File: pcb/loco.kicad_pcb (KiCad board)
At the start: 4 copper layers, 69.5 x 29.3 mm, 87 parts, among them J1 POWER, J2 INPUT, J3 I2C, J4 UART, J5 TagConnect, J6 GPIO_A, J7 GPIO_B, J8 Motor1, J9 Motor2, U1 NCV8718, U2 STM32G041K8U, U3 M95512-DRMF3TGK, U4 STSPIN220, U5 STSPIN220

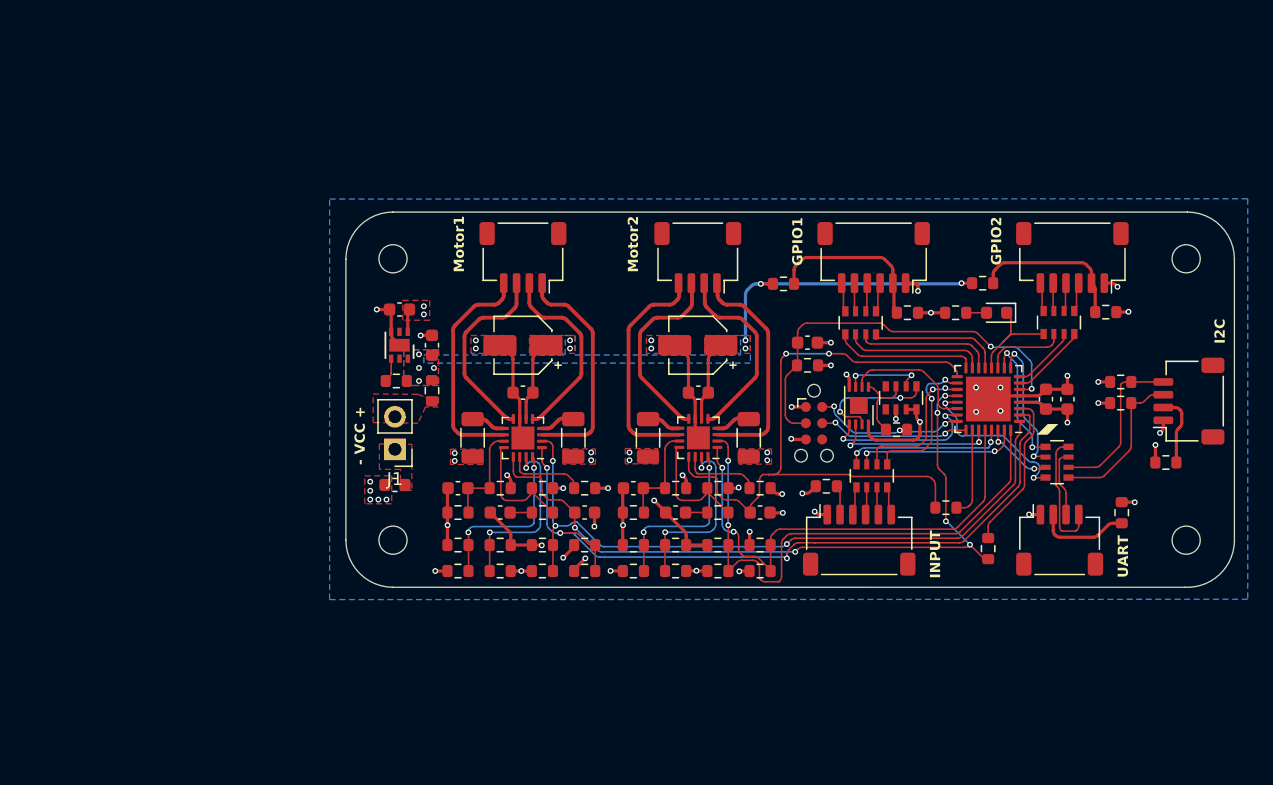
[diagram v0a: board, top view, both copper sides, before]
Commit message: pcb rev.0x03
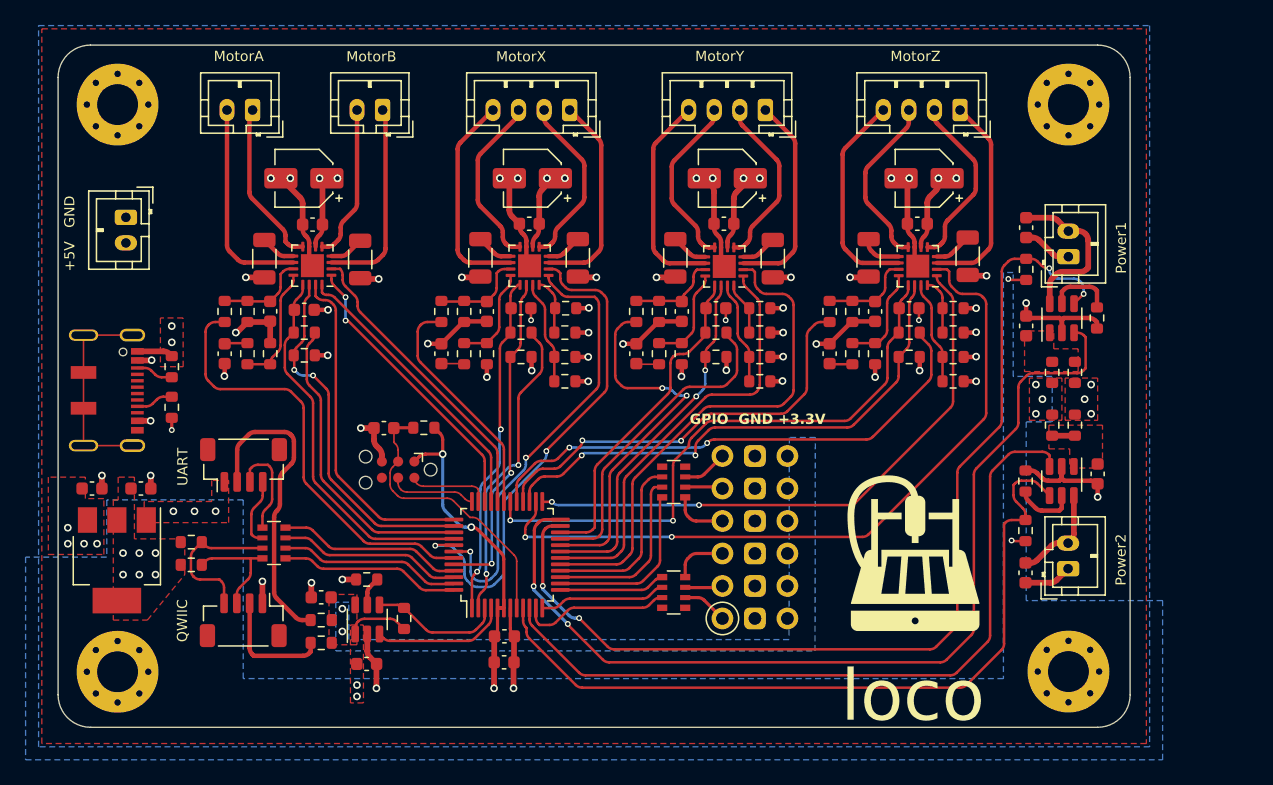
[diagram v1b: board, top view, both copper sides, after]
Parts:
- removed D1: LED, LED_SMD:LED_0603_1608Metric
- removed F1: Polyfuse, Fuse:Fuse_0603_1608Metric
- removed FB1, FB2, FB3, FB4, FB5, FB6: FerriteBead, Resistor_SMD:R_0603_1608Metric
- removed FB7, FB8: DNP, Resistor_SMD:R_0603_1608Metric
- removed J4: UART, Connector_JST:JST_SH_SM04B-SRSS-TB_1x04-1MP_P1.00mm_Horizontal
- removed J5: TagConnect, loco:Tag-Connect_TC2030-IDC-NL_2x03_P1.27mm_Vertical
- removed the REF** at (99.8, 56.3)
- removed RN4, RN5: 180Ω, Resistor_SMD:R_Array_Convex_4x0603
- added C16: 10uF, Capacitor_SMD:C_0603_1608Metric, F.Cu at (120.5, 59.1)
- added C17: 10uF, Capacitor_SMD:C_0603_1608Metric, F.Cu at (126.1, 70.7)
- added C18: 10uF, Capacitor_SMD:C_0603_1608Metric, F.Cu at (120.5, 51.4)
- added C19: 10uF, Capacitor_SMD:C_0603_1608Metric, F.Cu at (120.5, 78.4)
- added C20: 10uF, Capacitor_SMD:C_0603_1608Metric, F.Cu at (96.9, 51.1)
- added C21: 22uF, Capacitor_SMD:CP_Elec_4x4.5, F.Cu at (97.2, 47.6)
- added C22: 10uF, Capacitor_SMD:C_0603_1608Metric, F.Cu at (112.0, 51.1)
- added C23: 22uF, Capacitor_SMD:CP_Elec_4x4.5, F.Cu at (112.6, 47.6)
- added C24: 10uF, Capacitor_SMD:C_0603_1608Metric, F.Cu at (69.0, 85.5)
- added C25: 10uF, Capacitor_SMD:C_0603_1608Metric, F.Cu at (65.4, 80.3)
- added C26: 10uF, Capacitor_SMD:C_0603_1608Metric, F.Cu at (93.6, 58.0)
- added C27: 22nF, Capacitor_SMD:C_0603_1608Metric, F.Cu at (96.3, 57.7)
- added C28: 10uF, Capacitor_SMD:C_0603_1608Metric, F.Cu at (108.7, 58.0)
- added C29: 22nF, Capacitor_SMD:C_0603_1608Metric, F.Cu at (111.4, 57.7)
- added C30: 22nF, Capacitor_SMD:C_0603_1608Metric, F.Cu at (90.1, 61.3)
- added C31: 22nF, Capacitor_SMD:C_0603_1608Metric, F.Cu at (105.2, 61.3)
- added J10: Stepper1, Connector_JST:JST_PH_B4B-PH-K_1x04_P2.00mm_Vertical, F.Cu at (84.9, 42.2)
- added J11: Motor2, Connector_JST:JST_PH_B2B-PH-K_1x02_P2.00mm_Vertical, F.Cu at (60.1, 42.2)
- added J12: PWR1, Connector_JST:JST_PH_B2B-PH-K_1x02_P2.00mm_Vertical, F.Cu at (123.9, 53.7)
- added J13: PWR2, Connector_JST:JST_PH_B2B-PH-K_1x02_P2.00mm_Vertical, F.Cu at (123.8, 78.1)
- added J14: Stepper1, Connector_JST:JST_PH_B4B-PH-K_1x04_P2.00mm_Vertical, F.Cu at (100.2, 42.2)
- added J15: Stepper1, Connector_JST:JST_PH_B4B-PH-K_1x04_P2.00mm_Vertical, F.Cu at (115.4, 42.2)
- added R39: DNP, Resistor_SMD:R_0603_1608Metric, F.Cu at (99.7, 57.7)
- added R40: DNP, Resistor_SMD:R_0603_1608Metric, F.Cu at (114.8, 63.4)
- added R41: DNP, Resistor_SMD:R_0603_1608Metric, F.Cu at (114.8, 59.6)
- added R42: DNP, Resistor_SMD:R_0603_1608Metric, F.Cu at (114.8, 61.5)
- added R43: DNP, Resistor_SMD:R_0603_1608Metric, F.Cu at (114.8, 57.7)
- added R44: 10KΩ, Resistor_SMD:R_0603_1608Metric, F.Cu at (71.9, 82.0)
- added R45: 0.3Ω, Resistor_SMD:R_1206_3216Metric, F.Cu at (100.7, 53.9)
- added R46: 0.3Ω, Resistor_SMD:R_1206_3216Metric, F.Cu at (116.0, 53.7)
- added R47: 150KΩ, Resistor_SMD:R_0603_1608Metric, F.Cu at (69.0, 78.9)
- added R48: 10KΩ, Resistor_SMD:R_0603_1608Metric, F.Cu at (96.3, 59.6)
- added R49: 10KΩ, Resistor_SMD:R_0603_1608Metric, F.Cu at (111.4, 59.6)
- added R50: 0.3Ω, Resistor_SMD:R_1206_3216Metric, F.Cu at (93.1, 53.8)
- added R51: 0.3Ω, Resistor_SMD:R_1206_3216Metric, F.Cu at (108.2, 53.8)
- added R52: 10KΩ, Resistor_SMD:R_0603_1608Metric, F.Cu at (90.1, 58.0)
- added R53: 10KΩ, Resistor_SMD:R_0603_1608Metric, F.Cu at (105.2, 58.0)
- added R54: 47KΩ, Resistor_SMD:R_0603_1608Metric, F.Cu at (93.6, 61.3)
- added R55: 1KΩ, Resistor_SMD:R_0603_1608Metric, F.Cu at (91.8, 61.3)
- added R56: 47KΩ, Resistor_SMD:R_0603_1608Metric, F.Cu at (108.7, 61.3)
- added R57: 1KΩ, Resistor_SMD:R_0603_1608Metric, F.Cu at (107.0, 61.3)
- added R58: 1KΩ, Resistor_SMD:R_0603_1608Metric, F.Cu at (91.8, 58.0)
- added R59: 10KΩ, Resistor_SMD:R_0603_1608Metric, F.Cu at (96.3, 61.5)
- added R60: 1KΩ, Resistor_SMD:R_0603_1608Metric, F.Cu at (107.0, 58.0)
- added R61: 10KΩ, Resistor_SMD:R_0603_1608Metric, F.Cu at (111.4, 61.5)
- added REF**: OSHW-Logo_5.7x6mm_SilkScreen, Symbol:OSHW-Logo_5.7x6mm_SilkScreen, B.Cu at (111.6, 82.6)
- added U6: AP22652_3x, Package_TO_SOT_SMD:SOT-23-6, F.Cu at (123.3, 71.2)
- added U7: AP22652_3x, Package_TO_SOT_SMD:SOT-23-6, F.Cu at (69.0, 82.1)
- added U8: STSPIN220, Package_DFN_QFN:VQFN-16-1EP_3x3mm_P0.5mm_EP1.8x1.8mm, F.Cu at (96.9, 54.5)
- added U9: STSPIN220, Package_DFN_QFN:VQFN-16-1EP_3x3mm_P0.5mm_EP1.8x1.8mm, F.Cu at (112.1, 54.4)
- C1, C4, C8: value 1uF -> 10uF
- C11, C6: value 22nF -> 10uF
- C12: value 10uF -> 22nF
- C14, C15: value 22uF -> 22nF; footprint Capacitor_SMD:CP_Elec_4x4.5 -> Capacitor_SMD:C_0603_1608Metric
- C2: value 10uF -> 100nF
- C3: value 100nF -> 10uF
- C7: value 22nF -> 22uF; footprint Capacitor_SMD:C_0603_1608Metric -> Capacitor_SMD:CP_Elec_4x4.5
- C9: value 1uF -> 22uF; footprint Capacitor_SMD:C_0603_1608Metric -> Capacitor_SMD:CP_Elec_4x4.5
- H1, H2, H3, H4: footprint MountingHole:MountingHole_2.2mm_M2 -> MountingHole:MountingHole_3.2mm_M3_Pad_Via
- J1: value POWER -> I2C; footprint Connector_PinHeader_2.54mm:PinHeader_1x02_P2.54mm_Vertical -> Connector_JST:JST_SH_BM04B-SRSS-TB_1x04-1MP_P1.00mm_Vertical
- J2: value INPUT -> EXT; footprint Connector_JST:JST_SH_SM06B-SRSS-TB_1x06-1MP_P1.00mm_Horizontal -> Connector_JST:JST_PH_B2B-PH-K_1x02_P2.00mm_Vertical
- J3: value I2C -> GPIO; footprint Connector_JST:JST_SH_SM04B-SRSS-TB_1x04-1MP_P1.00mm_Horizontal -> Library:Header_03x06_P2.54mm_Vertical
- J6: value GPIO_A -> USB_C_Receptacle_USB2.0; footprint Connector_JST:JST_SH_SM06B-SRSS-TB_1x06-1MP_P1.00mm_Horizontal -> @jb:USB_C_Receptacle_JAE_DX07S016JA3R1500
- J7: value GPIO_B -> UART; footprint Connector_JST:JST_SH_SM06B-SRSS-TB_1x06-1MP_P1.00mm_Horizontal -> Connector_JST:JST_SH_BM04B-SRSS-TB_1x04-1MP_P1.00mm_Vertical
- J8: value Motor1 -> TagConnect; footprint Connector_JST:JST_SH_SM04B-SRSS-TB_1x04-1MP_P1.00mm_Horizontal -> Connector:Tag-Connect_TC2030-IDC-NL_2x03_P1.27mm_Vertical
- J9: value Motor2 -> Motor1; footprint Connector_JST:JST_SH_SM04B-SRSS-TB_1x04-1MP_P1.00mm_Horizontal -> Connector_JST:JST_PH_B2B-PH-K_1x02_P2.00mm_Vertical
- R1, R11: value 10KΩ -> DNP
- R12: value 10KΩ -> 0.3Ω; footprint Resistor_SMD:R_0603_1608Metric -> Resistor_SMD:R_1206_3216Metric
- R13, R16: value DNP -> 0.3Ω; footprint Resistor_SMD:R_0603_1608Metric -> Resistor_SMD:R_1206_3216Metric
- R14, R15, R25, R7: value DNP -> 10KΩ
- R17: value 15KΩ -> 0.3Ω; footprint Resistor_SMD:R_0603_1608Metric -> Resistor_SMD:R_1206_3216Metric
- R18, R27, R28: value 1KΩ -> 10KΩ
- R19: value 15KΩ -> 10KΩ
- R20: value 1KΩ -> 47KΩ
- R21, R23: value DNP -> 1KΩ
- R22: value DNP -> 47KΩ
- R24, R26: value 10KΩ -> 1KΩ
- R29: value DNP -> 0Ω
- R31: value 47KΩ -> 10KΩ
- R32: value 47KΩ -> 0Ω
- R34: value DNP -> 150KΩ
- R35: value 0.3Ω -> 150KΩ; footprint Resistor_SMD:R_1206_3216Metric -> Resistor_SMD:R_0603_1608Metric
- R36, R37, R38: value 0.3Ω -> DNP; footprint Resistor_SMD:R_1206_3216Metric -> Resistor_SMD:R_0603_1608Metric
- R4: value 10KΩ -> 5.1KΩ
- R5: value DNP -> 5.1KΩ
- R6: value 1KΩ -> DNP
- RN1, RN2: value 180Ω -> 190Ω
- RN3: value 10KΩ -> 190Ω
- U1: value NCV8718 -> LD1117S33TR_SOT223; footprint Package_DFN_QFN:DFN-6-1EP_2x2mm_P0.65mm_EP1x1.6mm -> Package_TO_SOT_SMD:SOT-223-3_TabPin2
- U2: value STM32G041K8U -> STM32C031CxUx; footprint Package_DFN_QFN:UFQFPN-32-1EP_5x5mm_P0.5mm_EP3.5x3.5mm -> Package_QFP:LQFP-48_7x7mm_P0.5mm
- U3: value M95512-DRMF3TGK -> STSPIN240; footprint Package_DFN_QFN:WDFN-8-1EP_3x2mm_P0.5mm_EP1.3x1.4mm -> Package_DFN_QFN:VQFN-16-1EP_3x3mm_P0.5mm_EP1.8x1.8mm
- U5: value STSPIN220 -> AP22652_3x; footprint Package_DFN_QFN:VQFN-16-1EP_3x3mm_P0.5mm_EP1.8x1.8mm -> Package_TO_SOT_SMD:SOT-23-6
- moved H4 84.2 mm to (49.5, 86.2)
- moved R3 73.8 mm to (55.3, 77.8)
- moved R2 73.7 mm to (55.3, 76.0)
- moved C3 71.1 mm to (51.3, 71.8), turned to 0 degrees
- moved J7 66.8 mm to (59.4, 70.0), turned to 0 degrees
- moved H2 62.8 mm to (123.9, 41.8)
- moved J2 62.6 mm to (50.2, 50.6), turned to -90 degrees
- moved RN2 61.6 mm to (61.7, 76.1)
- moved J6 59.6 mm to (49.9, 64.2), turned to -90 degrees
- moved R5 56.9 mm to (53.7, 62.3), turned to -90 degrees
- moved R6 55.1 mm to (65.4, 82.1)
- moved R4 49.8 mm to (53.7, 65.5), turned to -90 degrees
- moved R12 49.7 mm to (68.5, 53.9), turned to 90 degrees
- moved C2 47.8 mm to (79.8, 83.4), turned to 0 degrees
- moved C7 44.2 mm to (64.1, 47.6), turned to 180 degrees
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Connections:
- C1 pad 1: VCC -> VDD
- C10 pad 1: Net-(C10-Pad1) -> /M_FAULT
- C11 pad 1: Net-(C11-Pad1) -> Net-(U3-REF)
- C12 pad 1: VCC -> Net-(C12-Pad1)
- C13 pad 1: VCC -> Net-(U4-REF)
- C14 pad 1: VCC -> /S1_FAULT
- C15 pad 1: VCC -> Net-(C15-Pad1)
- C4 pad 1: VDD -> VCC
- C6 pad 1: /M1_FLT -> VCC
- C7 pad 1: /M2_FLT -> VCC
- C8 pad 1: Net-(U4-REF) -> VCC
- C9 pad 1: Net-(U5-REF) -> VCC
- J1 pad 1: /EXT_GND -> GND
- J1 pad 2: /EXT_PWR -> Net-(J1-Pin_2)
- J2 pad 2: /INPUT_VDD -> VCC
- J3 pad 1: GND -> Net-(J3-Pin_1)
- J3 pad 2: /I2C_VDD -> Net-(J3-Pin_2)
- J7 pad 2: /GPIO_B_VDD -> Net-(J7-Pin_2)
- J8 pad 1: /M1A1 -> VDD
- J8 pad 2: /M1A2 -> Net-(J8-Pin_2)
- J8 pad 3: /M1B2 -> /RESET
- J8 pad 4: /M1B1 -> Net-(J8-Pin_4)
- J9 pad 1: /M2A1 -> /M_A1
- J9 pad 2: /M2A2 -> /M_A2
- R1 pad 1: VCC -> Net-(J1-Pin_2)
- R1 pad 2: Net-(U1-EN) -> /GPIO_PWR 
- R10 pad 1: GND -> VCC
- R10 pad 2: Net-(U5-MODE2) -> Net-(U4-MODE2)
- R11 pad 1: /M1_EN -> Net-(U4-MODE1)
- R11 pad 2: /M1_FLT -> VCC
- R12 pad 1: /M2_EN -> GND
- R12 pad 2: /M2_FLT -> /M_S1
- R13 pad 2: Net-(U4-MODE1) -> /S1_S1
- R14 pad 1: GND -> /M_EN
- R14 pad 2: Net-(U5-MODE1) -> /M_FAULT
- R15 pad 1: Net-(U4-MODE1) -> /S1_EN
- R15 pad 2: VDD -> /S1_FAULT
- R16 pad 1: Net-(U5-MODE1) -> GND
- R16 pad 2: VDD -> /M_S2
- R17 pad 1: Net-(U4-REF) -> GND
- R17 pad 2: VDD -> /S1_S2
- R18 pad 1: Net-(U4-REF) -> /M_REF
- R18 pad 2: GND -> Net-(U3-REF)
- R19 pad 1: Net-(U5-REF) -> /S1_REF
- R19 pad 2: VDD -> Net-(U4-REF)
- R2 pad 2: Net-(J3-Pin_4) -> Net-(J1-Pin_4)
- R20 pad 1: Net-(U5-REF) -> Net-(U3-TOFF)
- R21 pad 1: GND -> Net-(U3-TOFF)
- R21 pad 2: /M1_STCK -> Net-(C12-Pad1)
- R22 pad 1: GND -> Net-(U4-TOFF)
- R22 pad 2: /M2_STCK -> GND
- R23 pad 1: /M1_STCK -> Net-(U4-TOFF)
- R23 pad 2: VDD -> Net-(C15-Pad1)
- R24 pad 1: VDD -> Net-(U3-REF)
- R24 pad 2: Net-(U4-STBY/RESET) -> GND
- R25 pad 1: /M2_STCK -> /M_STBY
- R25 pad 2: VDD -> GND
- R26 pad 1: VDD -> Net-(U4-REF)
- R26 pad 2: Net-(U5-STBY/RESET) -> GND
- R27 pad 1: Net-(U4-TOFF) -> /S1_STBY
- R27 pad 2: Net-(C10-Pad1) -> GND
- R28 pad 1: Net-(U5-TOFF) -> VDD
- R28 pad 2: Net-(C11-Pad1) -> /PWR2_SENSE
- R29 pad 1: GND -> VDD
- R29 pad 2: /M1_DIR -> Net-(U6-VIN)
- R3 pad 2: Net-(J3-Pin_3) -> Net-(J1-Pin_3)
- R30 pad 1: GND -> Net-(U6-VIN)
- R30 pad 2: /M2_DIR -> VCC
- R31 pad 1: Net-(U4-TOFF) -> VDD
- R31 pad 2: GND -> /PWR1_SENSE
- R32 pad 1: Net-(U5-TOFF) -> VDD
- R32 pad 2: GND -> Net-(U5-VIN)
- R33 pad 1: /M1_DIR -> Net-(U5-VIN)
- R33 pad 2: VDD -> VCC
- R34 pad 1: /M2_DIR -> GND
- R34 pad 2: VDD -> Net-(U5-ILIM)
- R35 pad 2: /M1S1 -> Net-(U6-ILIM)
- R36 pad 2: /M1S2 -> Net-(U8-MODE2)
- R37 pad 1: GND -> Net-(U8-MODE1)
- R37 pad 2: /M2S1 -> GND
- R38 pad 1: GND -> VCC
- R38 pad 2: /M2S2 -> Net-(U8-MODE2)
- R4 pad 1: VDD -> Net-(J6-CC2)
- R4 pad 2: /RESET -> GND
- R5 pad 1: Net-(RN3-R3.1) -> GND
- R5 pad 2: /SWDIO -> Net-(J6-CC1)
- R6 pad 1: VDD -> Net-(J7-Pin_2)
- R6 pad 2: Net-(D1-A) -> /GPIO_PWR 
- R7 pad 1: Net-(U4-MODE2) -> VDD
- R7 pad 2: VDD -> /RESET
- R8 pad 1: Net-(U5-MODE2) -> GND
- R8 pad 2: VDD -> Net-(U4-MODE2)
- R9 pad 1: GND -> Net-(U4-MODE1)
- R9 pad 2: Net-(U4-MODE2) -> GND
- RN1 pad 1: /ENC1 -> unconnected-(RN1-R1.1-Pad1)
- RN1 pad 2: /ENC2 -> Net-(J3-Pin_1)
- RN1 pad 3: /BTN2 -> Net-(J3-Pin_2)
- RN1 pad 4: /BTN1 -> Net-(J3-Pin_3)
- RN1 pad 5: Net-(J2-Pin_3) -> /GPIO3
- RN1 pad 6: Net-(J2-Pin_4) -> /GPIO2
- RN1 pad 7: Net-(J2-Pin_5) -> /GPIO1
- RN1 pad 8: Net-(J2-Pin_6) -> unconnected-(RN1-R1.2-Pad8)
- RN2 pad 1: Net-(J3-Pin_3) -> /I2C_SDA
- RN2 pad 2: Net-(J3-Pin_4) -> /I2C_SCL
- RN2 pad 3: Net-(J4-Pin_3) -> /UART_RX
- RN2 pad 4: Net-(J4-Pin_4) -> /UART_TX
- RN2 pad 5: /UART_RX -> Net-(J7-Pin_3)
- RN2 pad 6: /UART_TX -> Net-(J7-Pin_4)
- RN2 pad 7: /I2C_SCL -> Net-(J1-Pin_4)
- RN2 pad 8: /I2C_SDA -> Net-(J1-Pin_3)
- RN3 pad 1: Net-(RN3-R1.1) -> Net-(J3-Pin_4)
- RN3 pad 2: Net-(RN3-R2.1) -> Net-(J3-Pin_5)
- RN3 pad 3: Net-(RN3-R3.1) -> Net-(J3-Pin_6)
- RN3 pad 6: GND -> /GPIO6
- RN3 pad 7: VDD -> /GPIO5
- RN3 pad 8: VDD -> /GPIO4
- U1 pad 1: VDD -> GND
- U1 pad 2: unconnected-(U1-NC)_1 -> VDD
- U1 pad 3: GND -> VCC
- U2 pad 1: /M1_STCK -> /S1_FAULT
- U2 pad 10: /UART_RX -> /PWR2_SWITCH
- U2 pad 11: /GPIO7 -> /GPIO1
- U2 pad 12: /GPIO8 -> /GPIO2
- U2 pad 13: /GPIO1 -> /GPIO3
- U2 pad 14: /GPIO2 -> /GPIO4
- U2 pad 15: /GPIO3 -> /GPIO5
- U2 pad 16: /GPIO4 -> /GPIO6
- U2 pad 17: /M2_FLT -> /S2_STEP
- U2 pad 18: /ENC1 -> /S2_DIR
- U2 pad 19: /ENC2 -> /S2_STBY
- U2 pad 2: /M1_DIR -> /S1_EN
- U2 pad 20: /M1_FLT -> /S2_REF
- U2 pad 21: /I2C_SDA -> /S2_EN
- U2 pad 22: /SPI_MISO -> /S2_FAULT
- U2 pad 23: /SPI_MOSI -> /PWR1_SENSE
- U2 pad 24: /SWDIO -> /PWR1_SWITCH
- U2 pad 25: /SWDCLK -> /S3_DIR
- U2 pad 26: /M2_EN -> /S3_STEP
- U2 pad 27: /SPI_CLK -> /S3_STBY
- U2 pad 28: /M2_DIR -> /S3_REF
- U2 pad 29: /BTN1 -> /S3_EN
- U2 pad 3: /M1_EN -> /GPIO_PWR_SENSE
- U2 pad 30: /I2C_SCL -> /S3_FAULT
- U2 pad 31: /BTN2 -> /S1_REF
- U2 pad 32: /M2_STCK -> /M1_PWM
- U2 pad 33: GND -> /M2_PWM
- U2 pad 4: VDD -> /GPIO_PWR_SWITCH
- U2 pad 5: GND -> VDD
- U2 pad 6: /RESET -> VDD
- U2 pad 7: /GPIO5 -> GND
- U2 pad 8: /GPIO6 -> /RESET
- U2 pad 9: /UART_TX -> /PWR2_SENSE
- U3 pad 1: Net-(RN3-R3.1) -> /M1_PHASE
- U3 pad 2: /SPI_MISO -> /M1_PWM
- U3 pad 3: Net-(RN3-R2.1) -> /M_A1
- U3 pad 4: GND -> /M_S1
- U3 pad 5: /SPI_MOSI -> /M_A2
- U3 pad 6: /SPI_CLK -> VCC
- U3 pad 7: Net-(RN3-R1.1) -> GND
- U3 pad 8: VDD -> /M_B2
- U3 pad 9: (no net) -> /M_S2
- U4 pad 1: /M1_DIR -> /S1_DIR
- U4 pad 10: /M1B1 -> /S1_B1
- U4 pad 13: /M1_FLT -> /S1_FAULT
- U4 pad 14: Net-(U4-STBY/RESET) -> /S1_STBY
- U4 pad 2: /M1_STCK -> /S1_STEP
- U4 pad 3: /M1A1 -> /S1_A1
- U4 pad 4: /M1S1 -> /S1_S1
- U4 pad 5: /M1A2 -> /S1_A2
- U4 pad 8: /M1B2 -> /S1_B2
- U4 pad 9: /M1S2 -> /S1_S2
- U5 pad 1: /M2_DIR -> Net-(U5-VIN)
- U5 pad 2: /M2_STCK -> GND
- U5 pad 3: /M2A1 -> /PWR1_SWITCH
- U5 pad 4: /M2S1 -> /PWR1_SENSE
- U5 pad 5: /M2A2 -> Net-(U5-ILIM)
- U5 pad 6: VCC -> Net-(J12-Pin_2)
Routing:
- net /PWR1_SENSE: track 0.00 -> 79.6 mm, vias 0 -> 4
- net /PWR1_SWITCH: track 0.00 -> 74.7 mm, vias 0 -> 2
- net GND: track 65.3 -> 131.7 mm, vias 43 -> 54
- net /PWR2_SENSE: track 0.00 -> 60.3 mm
- net /PWR2_SWITCH: track 0.00 -> 59.1 mm
- net /M1_DIR: track 58.4 -> 0.00 mm, vias 3 -> 0
- net /S3_STEP: track 0.00 -> 57.4 mm, vias 0 -> 2
- net /M1_FLT: track 56.7 -> 0.00 mm, vias 6 -> 0
- net /M1_STCK: track 54.6 -> 0.00 mm, vias 3 -> 0
- net /M2_FLT: track 51.3 -> 0.00 mm, vias 2 -> 0
- net /S3_FAULT: track 0.00 -> 46.4 mm, vias 0 -> 2
- net /S3_DIR: track 0.00 -> 45.9 mm, vias 0 -> 2
- net /M2_STCK: track 43.4 -> 0.00 mm, vias 2 -> 0
- net /S3_STBY: track 0.00 -> 41.7 mm, vias 0 -> 2
- net /S3_EN: track 0.00 -> 41.0 mm, vias 0 -> 2
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- added copper zone on B.Cu, net /GPIO_PWR 
- added copper zone on F.Cu, net /GPIO_PWR 
- added copper zone on F.Cu, net Net-(U5-VIN)
- added copper zone on F.Cu, net Net-(U6-VIN)
- removed copper zone on F.Cu, net /EXT_GND
- removed copper zone on F.Cu, net /EXT_PWR
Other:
- board size 69.5 x 29.3 mm -> 83.8 x 53.3 mm
- board text added: "+5V GND"
- board text added: "GPIO GND +3.3V"
- board text added: "MotorA"
- board text added: "MotorB"
- board text added: "MotorX"
- board text added: "MotorY"
- board text added: "MotorZ"
- board text added: "Power1"
- board text added: "Power2"
- board text added: "QWIIC"
- board text added: "loco"
- board text added: "vitaly.codes/loco rev. 0x03"
- board text removed: "- VCC +"
- board text removed: "GPIO1"
- board text removed: "GPIO2"
- board text removed: "I2C"
- board text removed: "INPUT"
- board text removed: "Motor1"
- board text removed: "Motor2"
- board text removed: "vitaly.codes/loco rev 0.2"
- board text removed: "◢◤"
